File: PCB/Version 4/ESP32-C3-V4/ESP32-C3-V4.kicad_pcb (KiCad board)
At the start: 4 copper layers, 27.7 x 24.3 mm, 49 parts, among them J1 PH1257-WT-04, J2 DPS_PPS, Q1 SI2301CDS-T1-GE3, SW2 TS-1187A-B-A-B, U1 USB-C-16P-SMD, U2 DS8561-33S5, U3 ESP32-C3, U4 TC4056A, U5 SKCL3130ME, Y1 40MHz_S3240000151040

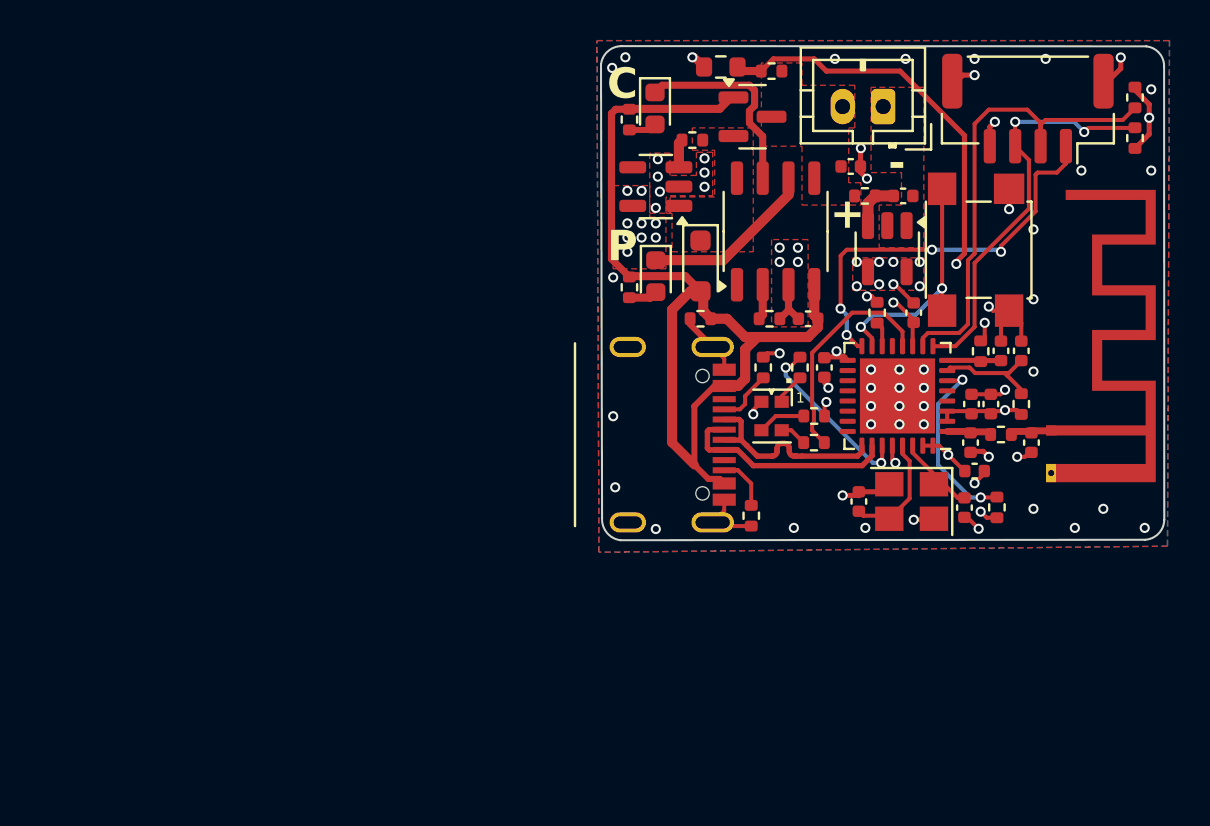
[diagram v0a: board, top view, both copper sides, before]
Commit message: Update Version 4 PCB and production outputs
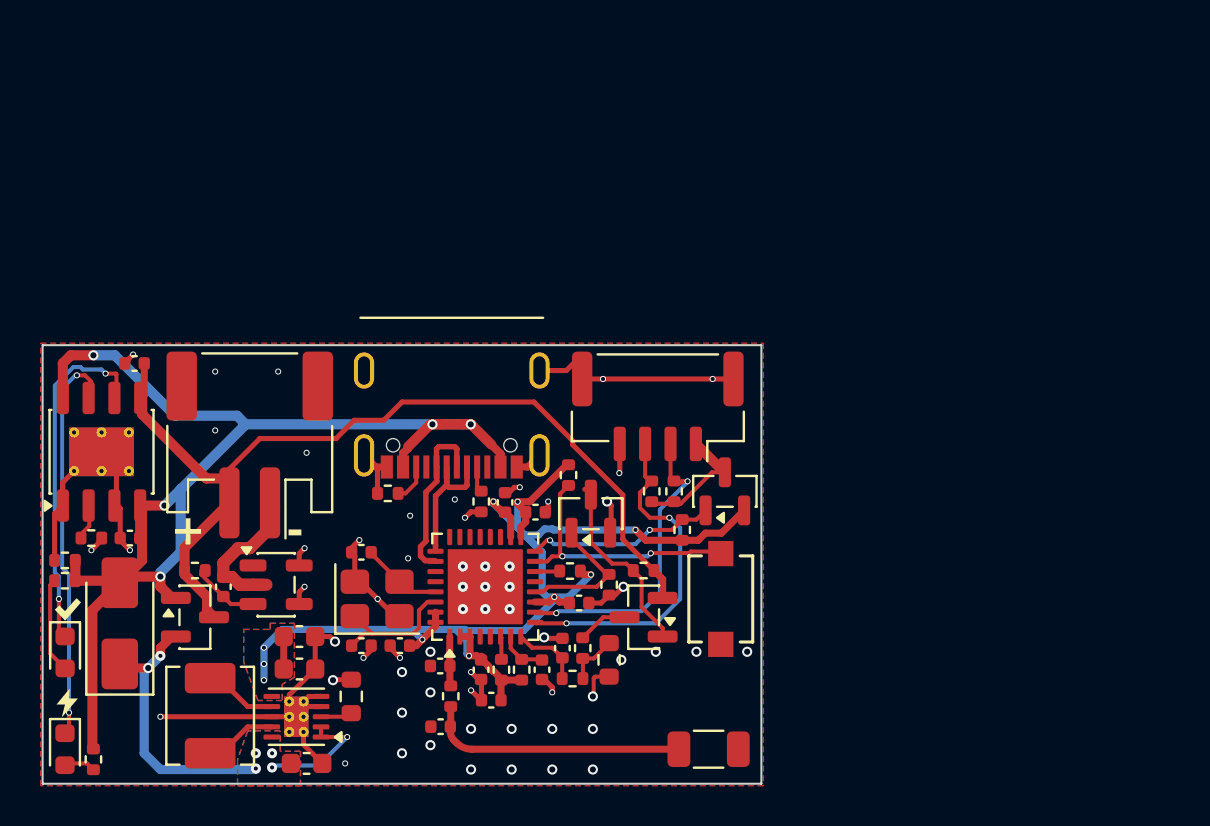
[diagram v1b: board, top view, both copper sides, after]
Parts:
- removed C11, C5, C7: 100n_0402_X7R_16V, Capacitor_SMD:C_0402_1005Metric
- removed C12: 15p_0402_C0G_50V, Capacitor_SMD:C_0402_1005Metric
- removed C3, C6: 3p3_0402_C0G_50V, Capacitor_SMD:C_0402_1005Metric
- removed D4: 1N5819WS(Basic), Diode_SMD:D_SOD-323_HandSoldering
- removed L1: 2n2H_0403_500mA, Resistor_SMD:R_0402_1005Metric
- removed R14: 2k0_0402, Resistor_SMD:R_0402_1005Metric
- removed U4: TC4056A, Package_SO:SOP-8_3.9x4.9mm_P1.27mm
- added C15: 22u_0603_X5R_6V3, Capacitor_SMD:C_0603_1608Metric, F.Cu at (114.2, 102.5)
- added C16: 100n_0402_X7R_16V, Capacitor_SMD:C_0402_1005Metric, F.Cu at (125.9, 94.8)
- added C17: 100n_0402_X7R_16V, Capacitor_SMD:C_0402_1005Metric, F.Cu at (119.2, 101.4)
- added C18: 3p3_0402_C0G_50V, Capacitor_SMD:C_0402_1005Metric, F.Cu at (121.2, 105.4)
- added C19: 3p3_0402_C0G_50V, Capacitor_SMD:C_0402_1005Metric, F.Cu at (121.2, 102.4)
- added C20: 10u_0402_X5R_6V3, Capacitor_SMD:C_0402_1005Metric, F.Cu at (123.7, 104.1)
- added C21: 100n_0402_X7R_16V, Capacitor_SMD:C_0402_1005Metric, F.Cu at (123.2, 102.6)
- added C22: 100n_0402_X7R_16V, Capacitor_SMD:C_0402_1005Metric, F.Cu at (128.0, 99.3)
- added C23: 100n_0402_X7R_16V, Capacitor_SMD:C_0402_1005Metric, F.Cu at (124.4, 94.3)
- added C25: 22u_0603_X5R_6V3, Capacitor_SMD:C_0603_1608Metric, F.Cu at (114.6, 107.2)
- added L2: 2u2_SL0420-2R2M, Inductor_SMD:L_Chilisin_BMRx00040412, F.Cu at (109.8, 104.8)
- added L3: 2n2H_0403_500mA, Resistor_SMD:R_0402_1005Metric, F.Cu at (121.7, 103.9)
- added Q3: SI2301CDS-T1-GE3, Package_TO_SOT_SMD:SOT-23, F.Cu at (131.2, 100.0)
- added Q4: 2N7002, Package_TO_SOT_SMD:SOT-23, F.Cu at (128.6, 94.9)
- added Q5: SI2301CDS-T1-GE3, Package_TO_SOT_SMD:SOT-23, F.Cu at (135.2, 93.8)
- added R17: 100k_0402, Resistor_SMD:R_0402_1005Metric, F.Cu at (127.7, 103.0)
- added R21: 4k7_0402, Resistor_SMD:R_0402_1005Metric, F.Cu at (104.1, 107.0)
- added U6: TPS63900DSKR, Package_SON:WSON-10-1EP_2.5x2.5mm_P0.5mm_EP1.2x2mm_ThermalVias, F.Cu at (114.1, 104.9)
- AE1: value KH-3216-H0209 -> ANT3216LL00R2400A; footprint RF_Antenna:Texas_SWRA117D_2.4GHz_Left -> Resistor_SMD:R_1206_3216Metric
- C1: value 100n_0402_X7R_16V -> 20p_0402_C0G_50V
- C10: value 15p_0402_C0G_50V -> 100n_0402_X7R_16V
- C13: value 100n_0402_X7R_16V -> 22u_0603_X5R_6V3; footprint Capacitor_SMD:C_0402_1005Metric -> Capacitor_SMD:C_0603_1608Metric
- C2: value 10u_0402_X5R_6V3 -> 20p_0402_C0G_50V
- D1: value XL-1615RGBC-RF -> M7(Basic); footprint LEDSMD:LED_0606_1432_correct -> Diode_SMD:D_SMA
- D3: value 0603_WHITE -> XL-1608UGC-04(Green)
- J1: value PH1257-WT-04 -> M1257RS-04P
- J2: value DPS_PPS -> BatConnect2PSMD; footprint Connector_JST:JST_PH_B2B-PH-K_1x02_P2.00mm_Vertical -> Connector_JST:JST_PH_S2B-PH-SM4-TB_1x02-1MP_P2.00mm_Horizontal
- R1, R6: value 10k_0402 -> 100k_0402
- R11: value 2k0_0402 -> 150k_0603; footprint Resistor_SMD:R_0402_1005Metric -> Resistor_SMD:R_0603_1608Metric
- R12: value 330_0402 -> 33k_0402
- R15: value 10k_0402 -> 1M_0402
- R18: value 1k_0402 -> 1M_0402
- R20: value 330k_0603 -> 4k7_0402; footprint Resistor_SMD:R_0603_1608Metric -> Resistor_SMD:R_0402_1005Metric
- R5: value 1k_0402 -> 36k5_0603; footprint Resistor_SMD:R_0402_1005Metric -> Resistor_SMD:R_0603_1608Metric
- R7: value 330_0402 -> 1M_0402
- R8: value 330_0402 -> 100k_0402
- SW2: value TS-1187A-B-A-B -> TS-1088-AR02016; footprint switch:SW_SPST_TL3305B -> footprints:SW_TS-1088_XNP
- U2: value DS8561-33S5 -> ESP32-C3; footprint Package_TO_SOT_SMD:SOT-23-5 -> Package_DFN_QFN:QFN-32-1EP_5x5mm_P0.5mm_EP3.7x3.7mm
- U3: value ESP32-C3 -> TP4056-42-ESOP8; footprint Package_DFN_QFN:QFN-32-1EP_5x5mm_P0.5mm_EP3.7x3.7mm -> Package_SO:HTSOP-8-1EP_3.9x4.9mm_P1.27mm_EP2.4x3.2mm_ThermalVias
- moved D2 42.9 mm to (102.7, 106.5)
- moved R20 41.0 mm to (102.7, 98.2), turned to 0 degrees
- moved U3 39.3 mm to (104.5, 91.8), turned to 90 degrees
- moved C4 38.6 mm to (110.5, 98.5), turned to 90 degrees
- moved R4 37.8 mm to (109.1, 97.7)
- moved R12 37.4 mm to (102.7, 97.2), turned to 180 degrees
- moved C13 37.3 mm to (114.2, 101.0), turned to 0 degrees
- moved Q1 36.9 mm to (109.1, 100.0)
- moved C9 36.6 mm to (106.1, 87.5), turned to 180 degrees
- moved J2 35.4 mm to (111.8, 91.5)
- moved R5 35.4 mm to (116.8, 103.9), turned to 90 degrees
- moved C8 35.1 mm to (105.9, 96.1)
- moved R16 35.1 mm to (104.0, 96.1)
- moved D3 34.5 mm to (102.7, 101.7)
- moved U5 34.3 mm to (113.1, 98.4), turned to 0 degrees
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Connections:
- AE1 pad 2: GND -> unconnected-(AE1-B-Pad2)
- C1 pad 1: +3.3V -> GND
- C1 pad 2: GND -> Net-(U2-XTAL_N)
- C10 pad 1: Net-(U3-XTAL_P) -> ADC
- C13 pad 1: ADC -> +3.3V
- C2 pad 2: +3.3V -> Net-(U2-XTAL_P)
- D1 pad 1: Net-(D1-RK) -> V_LDO
- D1 pad 2: +3.3V -> VCC
- J1 pad 1: VCC_Sensor -> Net-(J1-Pin_1)
- R10 pad 1: +3.3V -> MCU_SCL
- R10 pad 2: MCU_SCL -> Net-(J1-Pin_1)
- R11 pad 1: VCC -> Net-(R11-Pad1)
- R11 pad 2: Net-(D2-A) -> GND
- R12 pad 1: Rot -> VCC
- R12 pad 2: Net-(D1-RK) -> GND
- R13 pad 1: +BATT -> Net-(Q3-D)
- R13 pad 2: Net-(R13-Pad2) -> Net-(R11-Pad1)
- R15 pad 1: VCC -> GND
- R15 pad 2: GND -> ADC_EN
- R16 pad 2: Net-(U4-PROG) -> Net-(U3-PROG)
- R18 pad 1: V_LDO -> SENSOR_PWR_EN
- R18 pad 2: Net-(U2-EN) -> +3.3V
- R20 pad 1: Net-(R13-Pad2) -> Net-(D3-A)
- R20 pad 2: GND -> VCC
- R5 pad 1: Net-(R13-Pad2) -> Net-(U6-CFG1)
- R5 pad 2: ADC -> GND
- R7 pad 1: Blau -> +BATT
- R7 pad 2: Net-(D1-BK) -> Net-(Q3-G)
- R8 pad 1: Grün -> +3.3V
- R8 pad 2: Net-(D1-GK) -> Net-(U2-GPIO9)
- R9 pad 1: +3.3V -> MCU_SDA
- R9 pad 2: MCU_SDA -> Net-(J1-Pin_1)
- SW2 pad 2: Net-(U3-GPIO9) -> Net-(U2-GPIO9)
- U2 pad 1: V_LDO -> Net-(U2-LNA_IN)
- U2 pad 2: GND -> +3.3V
- U2 pad 3: Net-(U2-EN) -> +3.3V
- U2 pad 5: +3.3V -> unconnected-(U2-XTAL_32K_N-Pad5)
- U3 pad 1: Net-(U3-LNA_IN) -> GND
- U3 pad 2: +3.3V -> Net-(U3-PROG)
- U3 pad 3: +3.3V -> GND
- U3 pad 4: unconnected-(U3-XTAL_32K_P-Pad4) -> VCC
- U3 pad 5: unconnected-(U3-XTAL_32K_N-Pad5) -> +BATT
- U3 pad 6: EXTI -> Net-(D3-K)
- U3 pad 7: CHIP_EN -> Net-(D2-K)
- U3 pad 8: ADC -> VCC
- U3 pad 9: MCU_SCL -> GND
- Y1 pad 1: Net-(U3-XTAL_P) -> Net-(U2-XTAL_P)
- Y1 pad 3: Net-(U3-XTAL_N) -> Net-(U2-XTAL_N)
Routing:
- net +3.3V: track 17.3 -> 63.1 mm, vias 17 -> 10
- net +BATT: track 0.00 -> 44.4 mm
- net GND: track 33.3 -> 64.8 mm, vias 70 -> 60
- net Net-(R13-Pad2): track 24.0 -> 0.00 mm, vias 2 -> 0
- net V_LDO: track 0.00 -> 20.4 mm, vias 0 -> 7
- net VCC_Sensor: track 20.1 -> 0.00 mm, vias 4 -> 0
- net VCC: track 48.1 -> 63.8 mm, vias 0 -> 5
- net Net-(U2-GPIO9): track 0.00 -> 13.1 mm, vias 0 -> 2
- net Net-(U3-GPIO9): track 12.0 -> 0.00 mm, vias 2 -> 0
- net Net-(AE1-A): track 1.89 -> 13.0 mm
- net Grün: track 11.1 -> 0.00 mm
- net Net-(D2-K): track 9.85 -> 19.7 mm, vias 0 -> 2
- net SENSOR_PWR_EN: track 0.00 -> 9.75 mm, vias 0 -> 2
- net Net-(Q3-G): track 0.00 -> 9.16 mm
- net MCU_SDA: track 23.9 -> 15.2 mm, vias 0 -> 2
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- added copper zone on B.Cu, net +3.3V
- added copper zone on In2.Cu, net GND
- added copper zone on B.Cu, net V_LDO
- removed copper zone on In2.Cu, net +3.3V
- removed copper zone on F.Cu, net +BATT
- removed copper zone on F.Cu, net Earth
- removed copper zone on B.Cu, net GND
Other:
- board size 27.7 x 24.3 mm -> 35.4 x 21.6 mm
- board text added: "A.S. V4 W-Charger 08.26"
- board text added: "Char."
- board text added: "GND SCL SDA 3V3"
- board text added: "Pow."
- board text removed: "A.S. V3 W-Charger 07.24"
- board text removed: "C"
- board text removed: "Charg"
- board text removed: "GND"
- board text removed: "P"
- board text removed: "Power"
- board text removed: "SCL"
- board text removed: "SDA"
- board text removed: "VCC"
